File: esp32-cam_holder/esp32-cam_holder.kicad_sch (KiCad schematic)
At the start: 5 parts, among them J1 RJ45_Shielded, J2 UART, U1 ESP32-CAM

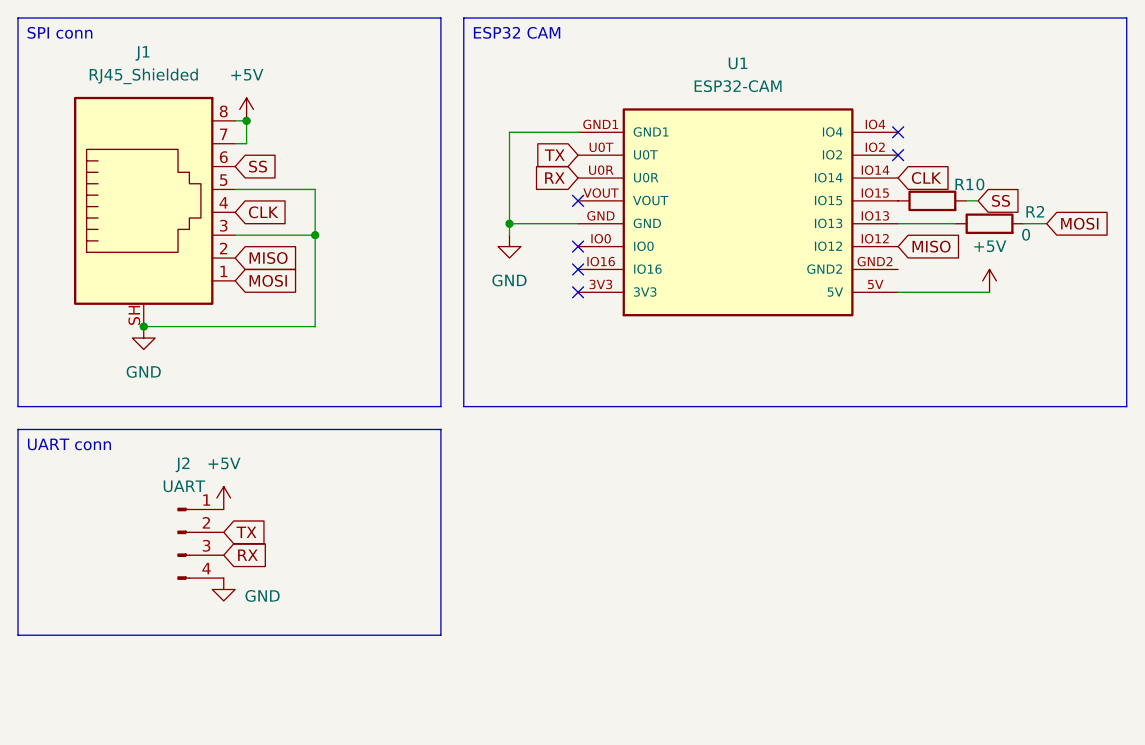
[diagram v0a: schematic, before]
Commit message: REV ALL
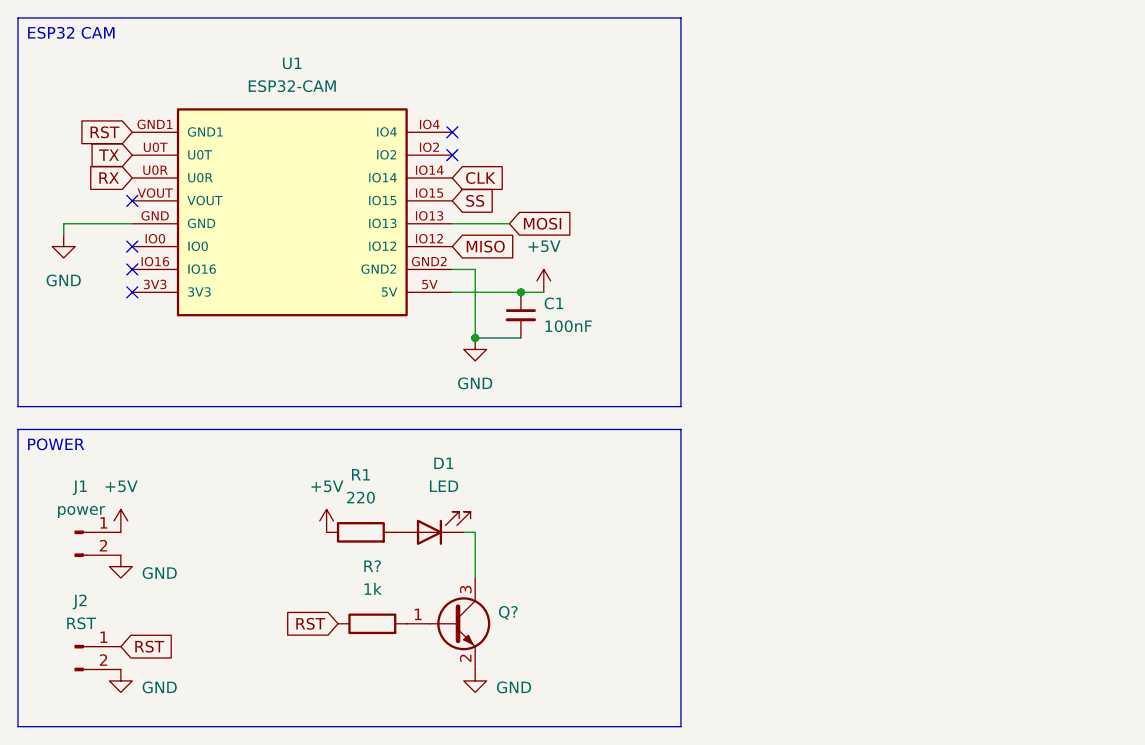
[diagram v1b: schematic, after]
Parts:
- removed J1: RJ45_Shielded, Connector_RJ:RJ45_Amphenol_RJHSE5380, symbol Connector:RJ45_Shielded
- removed J2: UART, Connector_PinHeader_2.54mm:PinHeader_1x04_P2.54mm_Horizontal, symbol Connector:Conn_01x04_Pin
- removed R2: 0, Resistor_SMD:R_1206_3216Metric_Pad1.30x1.75mm_HandSolder, symbol Device:R
- added C1: 100nF, Capacitor_SMD:C_0805_2012Metric_Pad1.18x1.45mm_HandSolder, symbol Device:C_Small
- added D1: LED, LED_THT:LED_D3.0mm_Horizontal_O1.27mm_Z10.0mm, symbol Device:LED
- added J1: power, Connector_JST:JST_XH_S2B-XH-A-1_1x02_P2.50mm_Horizontal, symbol Connector:Conn_01x02_Pin
- added J2: RST, Connector_JST:JST_XH_S2B-XH-A-1_1x02_P2.50mm_Horizontal, symbol Connector:Conn_01x02_Pin
- added Q?: MMBT3904, Package_TO_SOT_SMD:SOT-23, symbol Transistor_BJT:MMBT3904
- added R?: 1k, Resistor_SMD:R_0805_2012Metric_Pad1.20x1.40mm_HandSolder, symbol Device:R
- R1: value 0 -> 220; footprint Resistor_SMD:R_1206_3216Metric_Pad1.30x1.75mm_HandSolder -> Resistor_SMD:R_0805_2012Metric_Pad1.20x1.40mm_HandSolder
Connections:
- net +5V: now also R1.1, C1.1, J1.1 (Pin_1)
- net GND: now also U1.GND2, C1.2, J1.2 (Pin_2), J2.2 (Pin_2), Q?.2 (E); no longer U1.GND1
- net MOSI: now also U1.IO13
- net SS: now also U1.IO15; no longer R1.2
- new net: D1.2 (A), R1.2
- new net: Q?.1 (B), R?.2
- new net: D1.1 (K), Q?.3 (C)
- new net RST: J2.1 (Pin_1), R?.1, U1.GND1
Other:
- moved on the sheet: U1
